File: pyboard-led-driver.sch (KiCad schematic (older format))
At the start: 23 parts, among them J1 Ch1, J2 Ch2, J3 Ch3, P1 PYBD-WBUS-Host, U1 SN74AHCT125DR

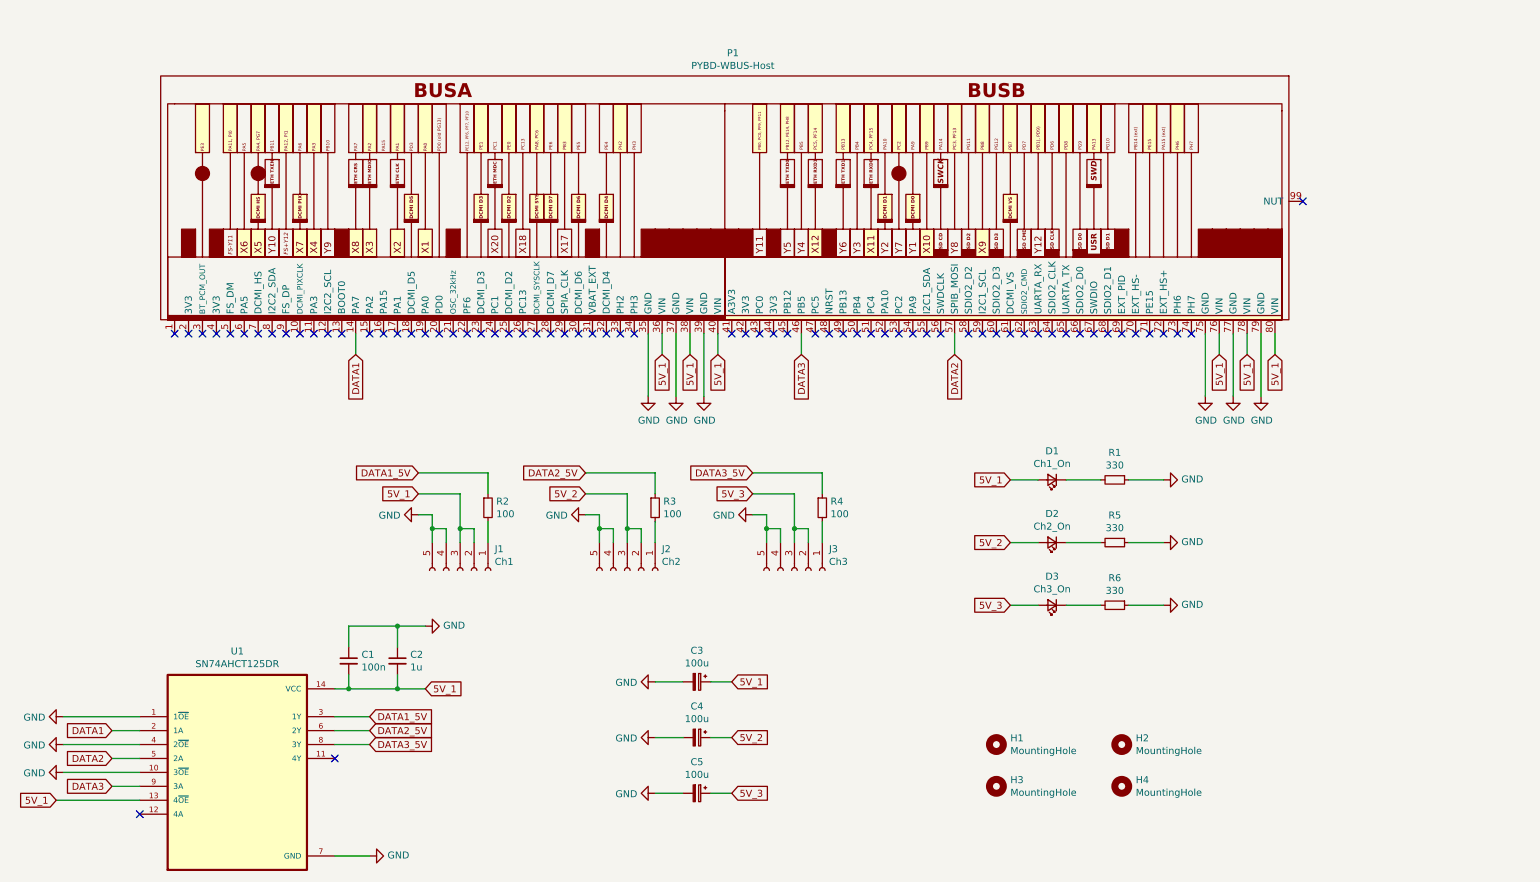
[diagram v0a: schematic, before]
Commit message: Board v1.0
Signed-off-by: Jim Mussared <jim.mussared@gmail.com>
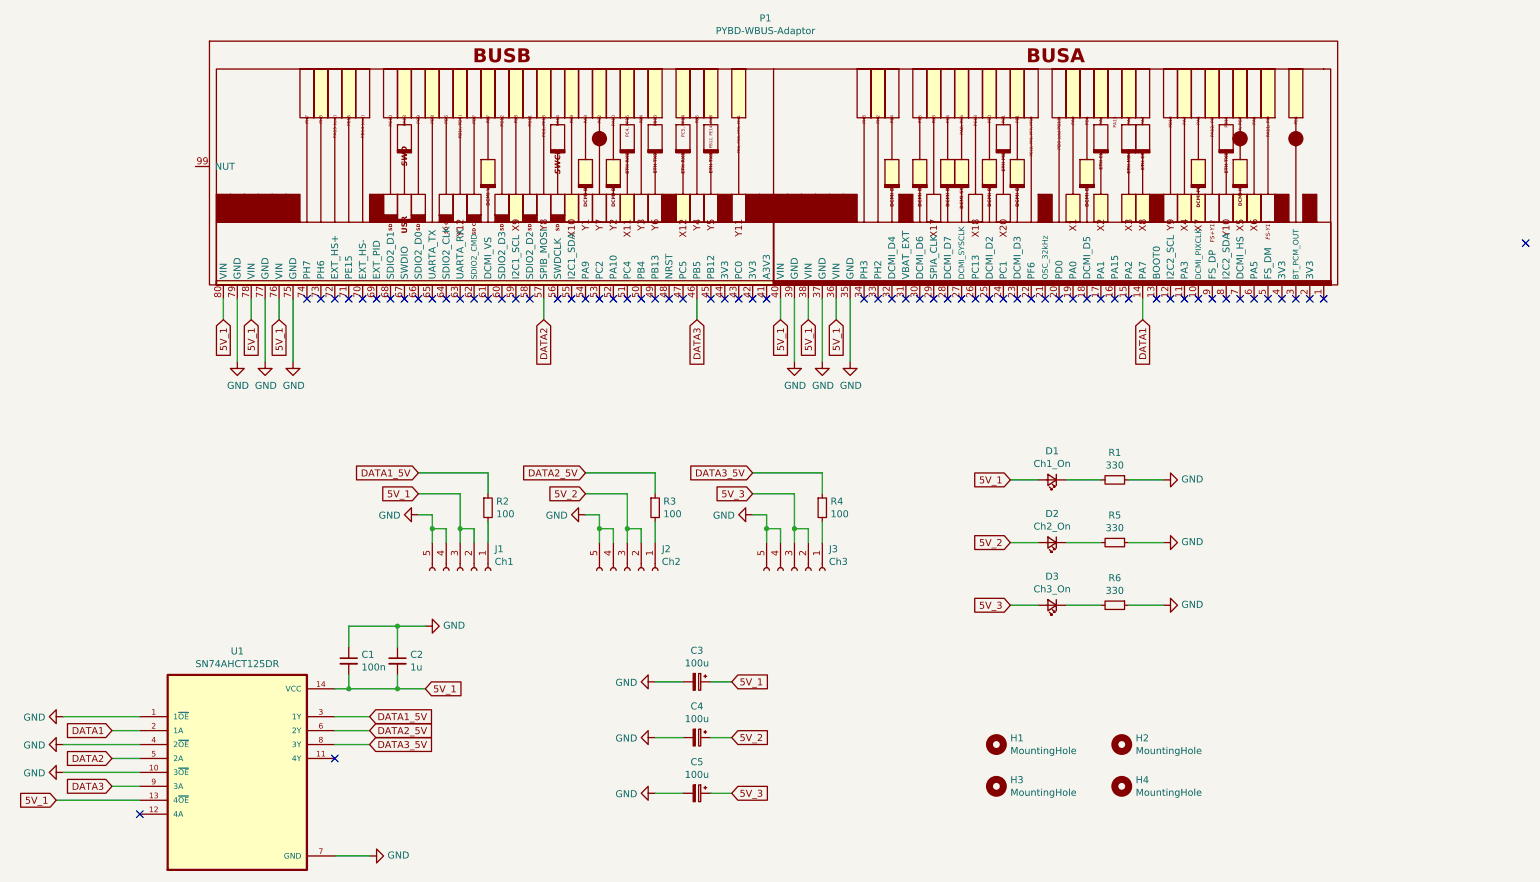
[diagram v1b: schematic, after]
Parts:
- removed P1: PYBD-WBUS-Host, MicroPython_Pyboard:PYBD_WBUS_Host, symbol MicroPython_Pyboard:PYBD-WBUS-Host
- added P1: PYBD-WBUS-Adaptor, MicroPython_Pyboard:PYBD_WBUS_Adaptor, symbol MicroPython_Pyboard:PYBD-WBUS-Adaptor
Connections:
- net 5V_1: now also P1.36 (VIN), P1.38 (VIN), P1.40 (VIN), P1.76 (VIN), P1.78 (VIN), P1.80 (VIN)
- net DATA1: now also P1.14 (PA7)
- net DATA2: now also P1.57 (SPIB_MOSI)
- net DATA3: now also P1.46 (PB5)
- net GND: now also P1.35 (GND), P1.37 (GND), P1.39 (GND), P1.75 (GND), P1.77 (GND), P1.79 (GND)
